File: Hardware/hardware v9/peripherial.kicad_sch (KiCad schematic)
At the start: 14 parts, among them J1 Micro_SD_Card_Det2

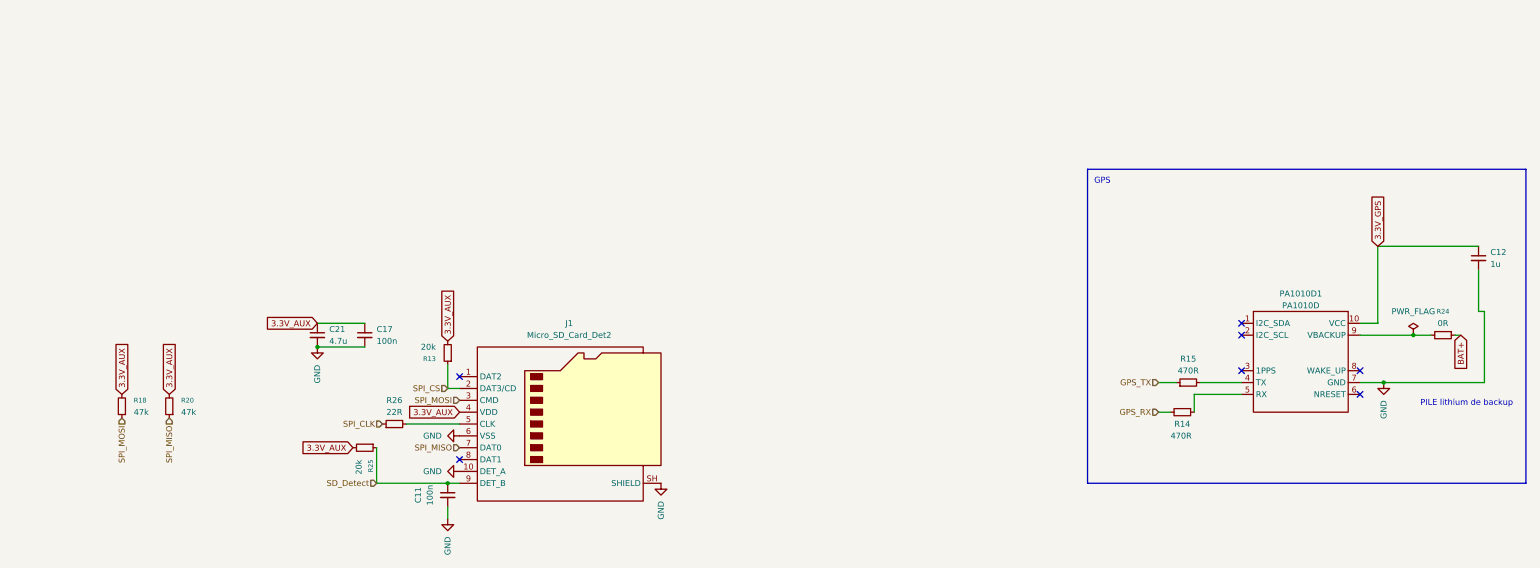
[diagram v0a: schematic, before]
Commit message: up
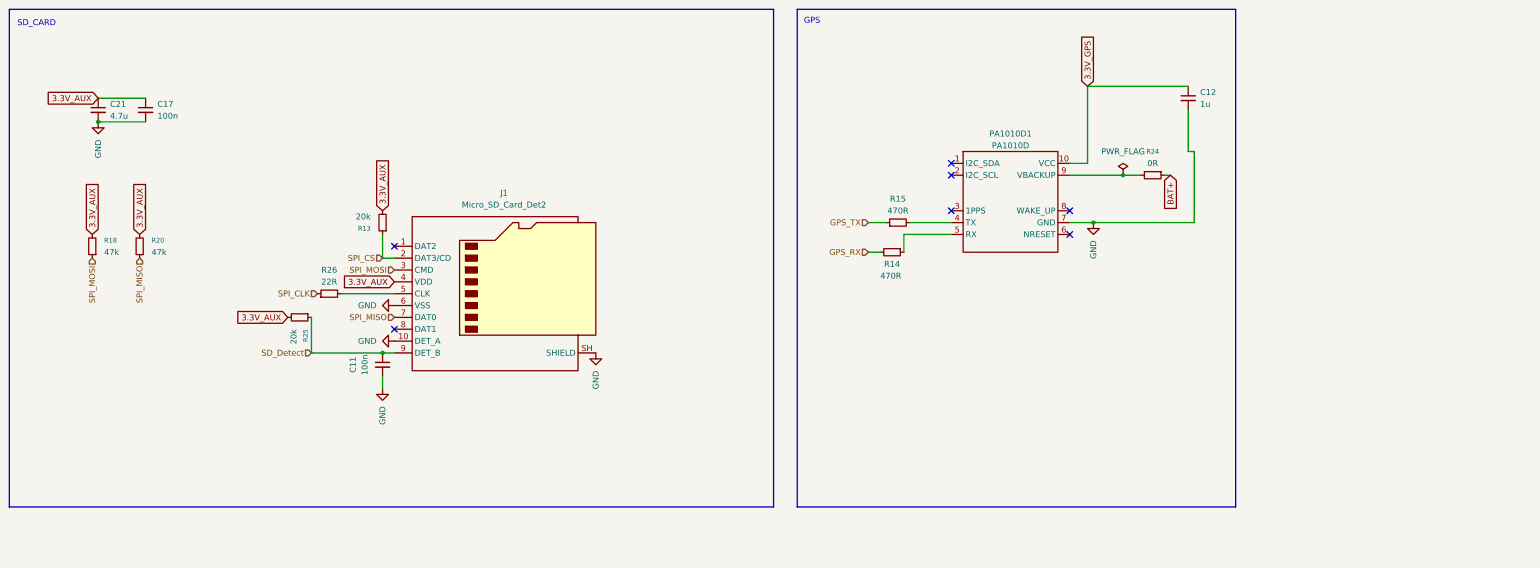
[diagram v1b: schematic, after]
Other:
- note added: "SD_CARD"
- note removed: "PILE lithium de backup"
- moved on the sheet: C11, C12, C17, C21, J1, PA1010D1, R13, R14, R15, R18, R20, R24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

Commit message: up
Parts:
- C11, C12, C17: footprint v9footprint:C_0201_0603Metric_Pad0.64x0.40mm_HandSolder -> v9footprintlocal:C_0201_0603Metric_Pad0.64x0.40mm_HandSolder
- C21: footprint v9footprint:C_0402_1005Metric -> v9footprintlocal:LED_0402_1005Metric
- J1: footprint v9footprint:microSD_HC_Molex_104031-0811 -> v9footprintlocal:microSD_HC_Molex_104031-0811
- PA1010D1: footprint v9footprint:PA1010D -> v9footprintlocal:PA1010D
- R13, R14, R15, R18, R20, R24, R25, R26: footprint v9footprint:R_0201_0603Metric_Pad0.64x0.40mm_HandSolder -> v9footprintlocal:R_0201_0603Metric_Pad0.64x0.40mm_HandSolder
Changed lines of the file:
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@@
 			)
 		)
-		(property "Footprint" "v9footprint:R_0201_0603Metric_Pad0.64x0.40mm_HandSolder"
+		(property "Footprint" "v9footprintlocal:R_0201_0603Metric_Pad0.64x0.40mm_HandSolder"
 			(at 81.28 74.93 0)
 			(hide yes)
@@
 			)
 		)
-		(property "Footprint" "v9footprint:C_0201_0603Metric_Pad0.64x0.40mm_HandSolder"
+		(property "Footprint" "v9footprintlocal:C_0201_0603Metric_Pad0.64x0.40mm_HandSolder"
 			(at 92.71 90.17 0)
 			(hide yes)
@@
 			)
 		)
-		(property "Footprint" "v9footprint:R_0201_0603Metric_Pad0.64x0.40mm_HandSolder"
+		(property "Footprint" "v9footprintlocal:R_0201_0603Metric_Pad0.64x0.40mm_HandSolder"
 			(at 92.71 59.69 0)
 			(hide yes)
@@
 			)
 		)
-		(property "Footprint" "v9footprint:PA1010D"
+		(property "Footprint" "v9footprintlocal:PA1010D"
 			(at 213.36 42.926 0)
 			(hide yes)
@@
 			)
 		)
-		(property "Footprint" "v9footprint:R_0201_0603Metric_Pad0.64x0.40mm_HandSolder"
+		(property "Footprint" "v9footprintlocal:R_0201_0603Metric_Pad0.64x0.40mm_HandSolder"
 			(at 201.93 66.04 0)
 			(hide yes)
@@
 			)
 		)
-		(property "Footprint" "v9footprint:C_0201_0603Metric_Pad0.64x0.40mm_HandSolder"
+		(property "Footprint" "v9footprintlocal:C_0201_0603Metric_Pad0.64x0.40mm_HandSolder"
 			(at 265.43 33.02 0)
 			(hide yes)
@@
 			)
 		)
-		(property "Footprint" "v9footprint:R_0201_0603Metric_Pad0.64x0.40mm_HandSolder"
+		(property "Footprint" "v9footprintlocal:R_0201_0603Metric_Pad0.64x0.40mm_HandSolder"
 			(at 257.81 49.53 0)
 			(hide yes)
@@
 			)
 		)
-		(property "Footprint" "v9footprint:R_0201_0603Metric_Pad0.64x0.40mm_HandSolder"
+		(property "Footprint" "v9footprintlocal:R_0201_0603Metric_Pad0.64x0.40mm_HandSolder"
 			(at 203.2 59.69 0)
 			(hide yes)
@@
 			)
 		)
-		(property "Footprint" "v9footprint:R_0201_0603Metric_Pad0.64x0.40mm_HandSolder"
+		(property "Footprint" "v9footprintlocal:R_0201_0603Metric_Pad0.64x0.40mm_HandSolder"
 			(at 40.64 64.77 0)
 			(hide yes)
@@
 			)
 		)
-		(property "Footprint" "v9footprint:R_0201_0603Metric_Pad0.64x0.40mm_HandSolder"
+		(property "Footprint" "v9footprintlocal:R_0201_0603Metric_Pad0.64x0.40mm_HandSolder"
 			(at 74.93 80.01 0)
 			(hide yes)
@@
 			)
 		)
-		(property "Footprint" "v9footprint:C_0201_0603Metric_Pad0.64x0.40mm_HandSolder"
+		(property "Footprint" "v9footprintlocal:C_0201_0603Metric_Pad0.64x0.40mm_HandSolder"
 			(at 41.91 35.56 0)
 			(hide yes)
@@
 			)
 		)
-		(property "Footprint" "v9footprint:R_0201_0603Metric_Pad0.64x0.40mm_HandSolder"
+		(property "Footprint" "v9footprintlocal:R_0201_0603Metric_Pad0.64x0.40mm_HandSolder"
 			(at 30.48 64.77 0)
 			(hide yes)
@@
 			)
 		)
-		(property "Footprint" "v9footprint:C_0402_1005Metric"
+		(property "Footprint" "v9footprintlocal:LED_0402_1005Metric"
 			(at 31.75 35.56 0)
 			(hide yes)
@@
 			)
 		)
-		(property "Footprint" "v9footprint:microSD_HC_Molex_104031-0811"
+		(property "Footprint" "v9footprintlocal:microSD_HC_Molex_104031-0811"
 			(at 170.18 57.15 0)
 			(hide yes)
